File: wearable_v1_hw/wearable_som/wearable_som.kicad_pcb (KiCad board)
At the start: 4 copper layers, 40.2 x 40 mm, 48 parts, among them IC1 TPS7A0228PDBVR, IC2 DA7280-00FV2, J1 Conn_01x04, J2 USB4105-GF-A, J3 Conn_01x03, M1 Motor_DC, Q1 PMOS, SW1 Reset, SW2 SW_Nidec_CAS-120A1, SW3 Boot, U1 STM32WB55RGVx, U2 BMI270, U3 MCP73831-2-MC, U4 DLF162500LT-5028A1, U5 2450AT18A100E, U6 USBLC6-2SC6, Y1 Crystal_GND23, Y2 Crystal

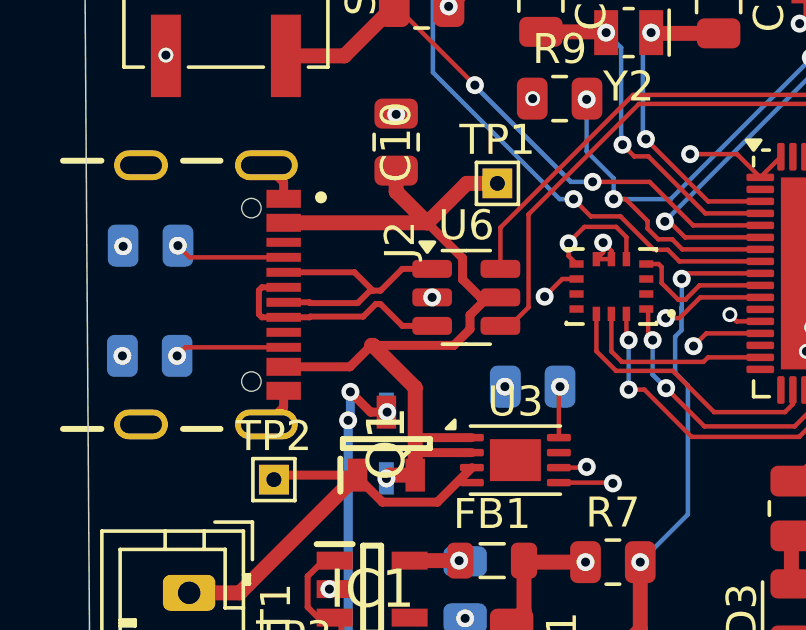
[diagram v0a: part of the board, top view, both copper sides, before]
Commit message: wearables v2
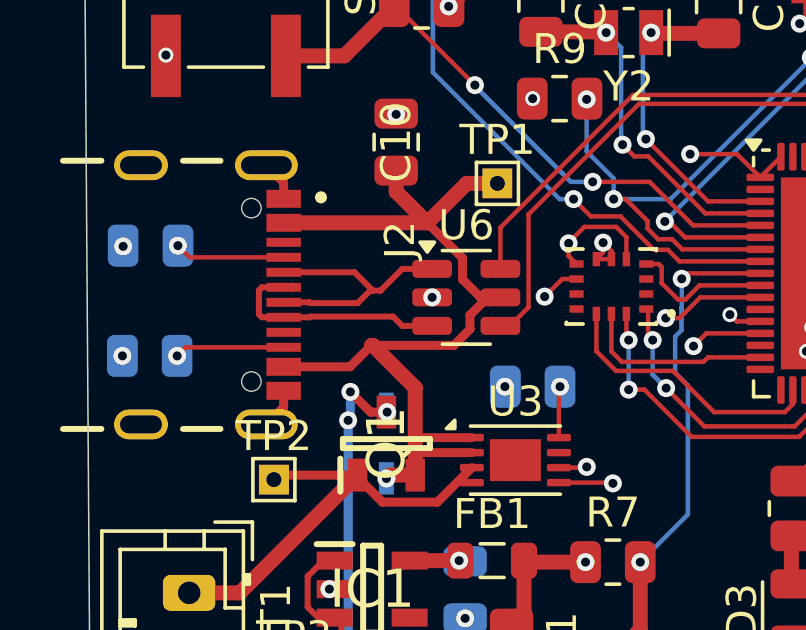
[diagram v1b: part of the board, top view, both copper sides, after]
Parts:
- C11: value 100nF -> 0.1uF
- C3: value 0.1u -> 0.1uF
- C4: value 1uF -> 0.1uF
